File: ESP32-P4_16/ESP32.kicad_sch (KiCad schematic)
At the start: 1 part, among them U1 ESP32-P4-ETH

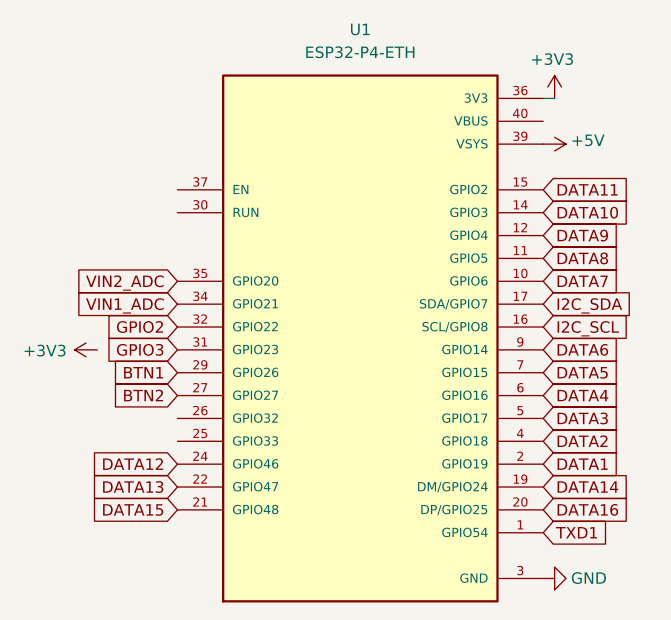
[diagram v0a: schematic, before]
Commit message: updates
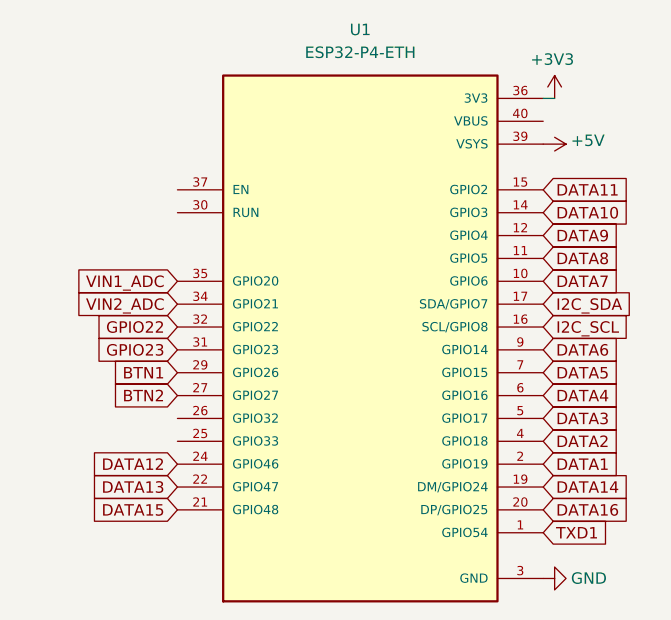
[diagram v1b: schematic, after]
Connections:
- net VIN1_ADC: now also U1.35 (GPIO20); no longer U1.34 (GPIO21)
- net VIN2_ADC: now also U1.34 (GPIO21); no longer U1.35 (GPIO20)
- net GPIO2 renamed GPIO22
- net GPIO3 renamed GPIO23
